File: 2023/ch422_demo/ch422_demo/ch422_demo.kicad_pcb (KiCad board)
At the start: 2 copper layers, 35 x 26 mm, 19 parts, among them J1 ch422, J2 hours, J3 minutes, J4 IIC_Conn

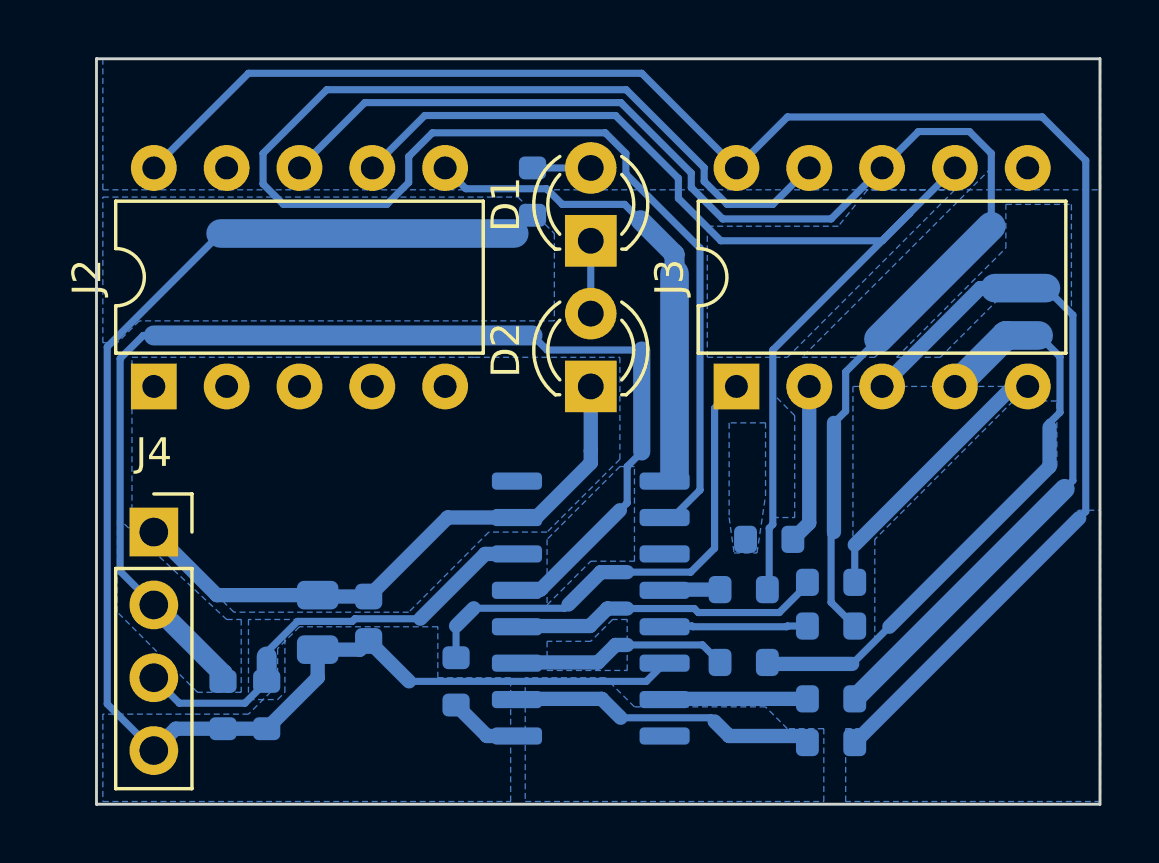
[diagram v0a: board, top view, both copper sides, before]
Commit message: forgot a few weekly commits.
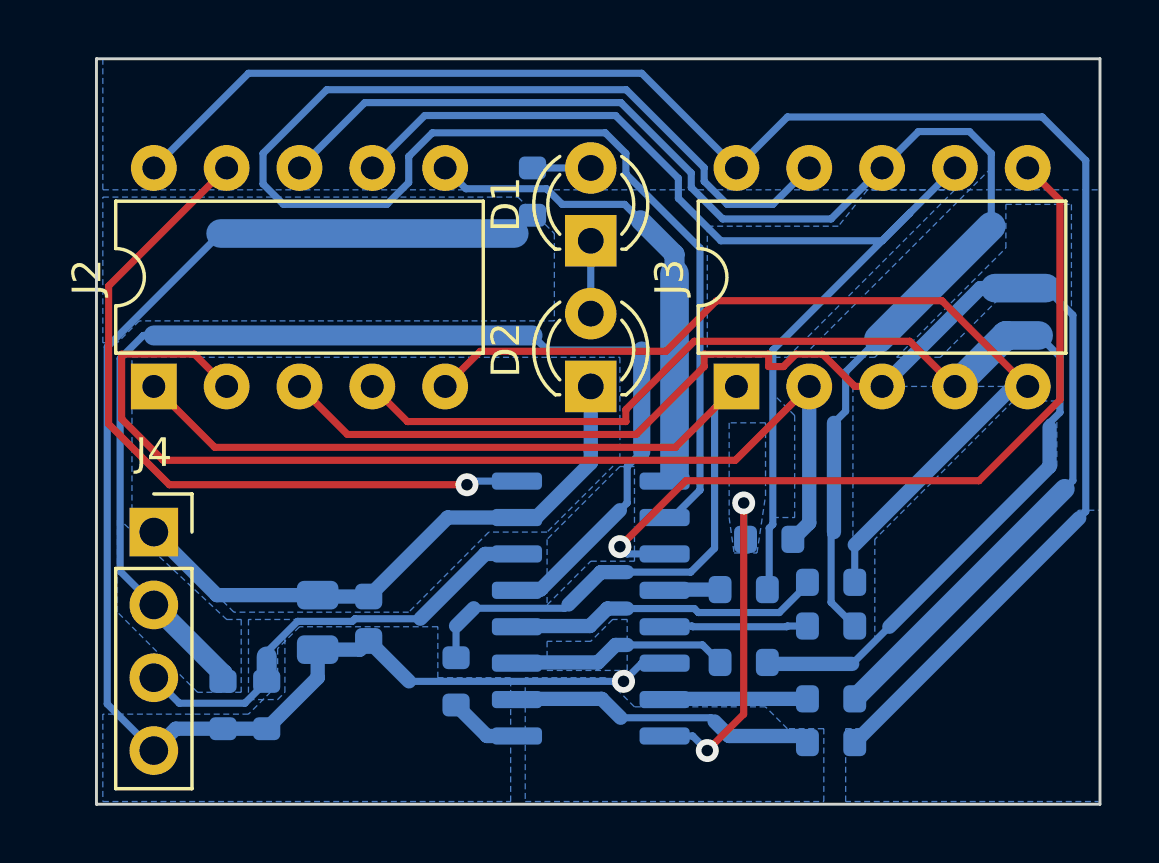
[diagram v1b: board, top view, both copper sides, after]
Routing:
- net /SEG_L_3: track 5.57 -> 37.6 mm
- net /DIG_3: track 0.00 -> 27.7 mm, vias 0 -> 1
- net /DIG_0: track 0.00 -> 25.8 mm, vias 0 -> 1
- net /SEG_L_2: track 25.0 -> 48.5 mm
- net /SEG_L_6: track 21.3 -> 44.2 mm
- net /SEG_L_7: track 9.12 -> 31.9 mm
- net /SEG_L_4: track 17.2 -> 39.3 mm
- net /SEG_3: track 0.00 -> 12.2 mm, vias 0 -> 2
- net VCC: vias 0 -> 1
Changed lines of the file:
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@@
   (gr_rect (start 33.56 17.02) (end 68.56 43.02)
     (stroke (width 0.1) (type default)) (fill none) (layer "Edge.Cuts"))
+  (via (at 51.943 38.735) (size 0.8) (drill 0.4) (layers "F.Cu" "B.Cu") (net 1))
   (segment (start 41.275 37.627853) (end 42.751 37.627853) (width 0.5) (layer "B.Cu") (net 1))
   (segment (start 44.462147 38.735) (end 43.053 37.325853) (width 0.5) (layer "B.Cu") (net 1))
-  (segment (start 52.74 38.735) (end 44.462147 38.735) (width 0.25) (layer "B.Cu") (net 1))
+  (segment (start 52.578 38.1) (end 51.943 38.735) (width 0.25) (layer "B.Cu") (net 1))
   (segment (start 33.935 27.068604) (end 33.935 39.523) (width 0.25) (layer "B.Cu") (net 1))
   (segment (start 36.322 40.386) (end 35.56 41.148) (width 0.5) (layer "B.Cu") (net 1))
-  (segment (start 53.375 38.1) (end 52.74 38.735) (width 0.25) (layer "B.Cu") (net 1))
   (segment (start 41.275 38.608) (end 41.275 37.627853) (width 0.5) (layer "B.Cu") (net 1))
   (segment (start 33.935 39.523) (end 35.56 41.148) (width 0.25) (layer "B.Cu") (net 1))
   (segment (start 42.751 37.627853) (end 43.053 37.325853) (width 0.5) (layer "B.Cu") (net 1))
+  (segment (start 51.943 38.735) (end 44.462147 38.735) (width 0.25) (layer "B.Cu") (net 1))
   (segment (start 37.889604 23.114) (end 33.935 27.068604) (width 0.25) (layer "B.Cu") (net 1))
   (segment (start 48.132 23.114) (end 37.889604 23.114) (width 1) (layer "B.Cu") (net 1))
@@
   (segment (start 39.497 40.386) (end 37.973 40.386) (width 0.5) (layer "B.Cu") (net 1))
   (segment (start 39.497 40.386) (end 41.275 38.608) (width 0.5) (layer "B.Cu") (net 1))
+  (segment (start 53.375 38.1) (end 52.578 38.1) (width 0.25) (layer "B.Cu") (net 1))
   (segment (start 48.225 33.02) (end 48.895 33.02) (width 0.5) (layer "B.Cu") (net 2))
   (segment (start 37.759853 35.727853) (end 35.56 33.528) (width 0.5) (layer "B.Cu") (net 2))
@@
   (segment (start 44.856147 36.550853) (end 47.117 34.29) (width 0.5) (layer "B.Cu") (net 10))
   (segment (start 39.497 38.736) (end 39.497 37.86768) (width 0.7) (layer "B.Cu") (net 10))
+  (segment (start 36.102604 31.877) (end 33.985 29.759396) (width 0.25) (layer "F.Cu") (net 11))
+  (segment (start 33.985 24.943) (end 38.1 20.828) (width 0.25) (layer "F.Cu") (net 11))
+  (segment (start 46.482 31.877) (end 36.102604 31.877) (width 0.25) (layer "F.Cu") (net 11))
+  (segment (start 33.985 29.759396) (end 33.985 24.943) (width 0.25) (layer "F.Cu") (net 11))
+  (via (at 46.482 31.877) (size 0.8) (drill 0.4) (layers "F.Cu" "B.Cu") (net 11))
+  (segment (start 46.609 31.75) (end 46.482 31.877) (width 0.25) (layer "B.Cu") (net 11))
+  (segment (start 48.225 31.75) (end 46.609 31.75) (width 0.25) (layer "B.Cu") (net 11))
   (segment (start 53.721 24.511) (end 53.721 23.839) (width 0.7) (layer "B.Cu") (net 12))
   (segment (start 49.260462 21.553) (end 49.805462 22.098) (width 0.25) (layer "B.Cu") (net 12))
@@
   (segment (start 39.37 20.32) (end 41.5908 18.0992) (width 0.25) (layer "B.Cu") (net 13))
   (segment (start 54.61 32.061751) (end 54.61 23.622) (width 0.25) (layer "B.Cu") (net 13))
+  (segment (start 51.816 34.036) (end 54.115 31.737) (width 0.25) (layer "F.Cu") (net 14))
+  (segment (start 54.115 31.737) (end 64.341991 31.737) (width 0.25) (layer "F.Cu") (net 14))
+  (segment (start 67.165 28.913991) (end 67.165 21.953) (width 0.25) (layer "F.Cu") (net 14))
+  (segment (start 67.165 21.953) (end 66.04 20.828) (width 0.25) (layer "F.Cu") (net 14))
+  (segment (start 64.341991 31.737) (end 67.165 28.913991) (width 0.25) (layer "F.Cu") (net 14))
+  (via (at 51.816 34.036) (size 0.8) (drill 0.4) (layers "F.Cu" "B.Cu") (net 14))
+  (segment (start 52.07 34.29) (end 51.816 34.036) (width 0.25) (layer "B.Cu") (net 14))
+  (segment (start 53.375 34.29) (end 52.07 34.29) (width 0.25) (layer "B.Cu") (net 14))
   (segment (start 53.375 35.534853) (end 55.309 35.534853) (width 0.5) (layer "B.Cu") (net 15))
   (segment (start 57.658 36.804853) (end 58.357 36.804853) (width 0.25) (layer "B.Cu") (net 16))
@@
   (segment (start 53.375 36.804853) (end 54.330853 36.804853) (width 0.25) (layer "B.Cu") (net 16))
   (segment (start 53.375 39.344853) (end 58.357 39.344853) (width 0.5) (layer "B.Cu") (net 17))
+  (segment (start 56.134 39.878) (end 56.134 32.512) (width 0.25) (layer "F.Cu") (net 18))
+  (segment (start 54.864 41.148) (end 56.134 39.878) (width 0.25) (layer "F.Cu") (net 18))
+  (via (at 54.864 41.148) (size 0.8) (drill 0.4) (layers "F.Cu" "B.Cu") (net 18))
+  (via (at 56.134 32.512) (size 0.8) (drill 0.4) (layers "F.Cu" "B.Cu") (net 18))
+  (segment (start 56.134 33.718) (end 56.198 33.782) (width 0.25) (layer "B.Cu") (net 18))
+  (segment (start 53.375 40.64) (end 54.356 40.64) (width 0.25) (layer "B.Cu") (net 18))
+  (segment (start 56.134 32.512) (end 56.134 33.718) (width 0.25) (layer "B.Cu") (net 18))
+  (segment (start 54.356 40.64) (end 54.864 41.148) (width 0.25) (layer "B.Cu") (net 18))
+  (segment (start 55.88 28.448) (end 53.755 30.573) (width 0.25) (layer "F.Cu") (net 19))
+  (segment (start 53.755 30.573) (end 37.685 30.573) (width 0.25) (layer "F.Cu") (net 19))
+  (segment (start 37.685 30.573) (end 35.56 28.448) (width 0.25) (layer "F.Cu") (net 19))
   (segment (start 52.07 34.925) (end 54.286751 34.925) (width 0.25) (layer "B.Cu") (net 19))
   (segment (start 46.717125 36.185) (end 49.893249 36.185) (width 0.25) (layer "B.Cu") (net 19))
@@
   (segment (start 46.101 37.91) (end 46.101 36.801125) (width 0.25) (layer "B.Cu") (net 19))
   (segment (start 55.118 29.21) (end 55.88 28.448) (width 0.25) (layer "B.Cu") (net 19))
+  (segment (start 38.1 28.448) (end 36.975 27.323) (width 0.25) (layer "F.Cu") (net 20))
+  (segment (start 34.435 29.573) (end 35.885 31.023) (width 0.25) (layer "F.Cu") (net 20))
+  (segment (start 35.885 31.023) (end 55.845 31.023) (width 0.25) (layer "F.Cu") (net 20))
+  (segment (start 55.845 31.023) (end 58.42 28.448) (width 0.25) (layer "F.Cu") (net 20))
+  (segment (start 34.435 27.323) (end 34.435 29.573) (width 0.25) (layer "F.Cu") (net 20))
+  (segment (start 36.975 27.323) (end 34.435 27.323) (width 0.25) (layer "F.Cu") (net 20))
   (segment (start 58.42 28.448) (end 58.42 33.21) (width 0.5) (layer "B.Cu") (net 20))
   (segment (start 58.42 33.21) (end 57.848 33.782) (width 0.5) (layer "B.Cu") (net 20))
+  (segment (start 60.010991 28.448) (end 60.96 28.448) (width 0.25) (layer "F.Cu") (net 21))
+  (segment (start 57.954009 27.323) (end 58.885991 27.323) (width 0.25) (layer "F.Cu") (net 21))
+  (segment (start 52.387 30.123) (end 54.755 27.755) (width 0.25) (layer "F.Cu") (net 21))
+  (segment (start 58.885991 27.323) (end 60.010991 28.448) (width 0.25) (layer "F.Cu") (net 21))
+  (segment (start 57.005 27.323) (end 57.005 27.755) (width 0.25) (layer "F.Cu") (net 21))
+  (segment (start 57.005 27.755) (end 57.522009 27.755) (width 0.25) (layer "F.Cu") (net 21))
+  (segment (start 54.755 27.323) (end 57.005 27.323) (width 0.25) (layer "F.Cu") (net 21))
+  (segment (start 57.522009 27.755) (end 57.954009 27.323) (width 0.25) (layer "F.Cu") (net 21))
+  (segment (start 40.64 28.448) (end 42.315 30.123) (width 0.25) (layer "F.Cu") (net 21))
+  (segment (start 54.755 27.755) (end 54.755 27.323) (width 0.25) (layer "F.Cu") (net 21))
+  (segment (start 42.315 30.123) (end 52.387 30.123) (width 0.25) (layer "F.Cu") (net 21))
   (segment (start 64.389 25.019) (end 60.96 28.448) (width 0.5) (layer "B.Cu") (net 21))
   (segment (start 67.615 31.736853) (end 67.615 25.959) (width 0.25) (layer "B.Cu") (net 21))
@@
   (segment (start 67.615 25.959) (end 66.675 25.019) (width 0.25) (layer "B.Cu") (net 21))
   (segment (start 64.897 25.019) (end 64.389 25.019) (width 0.5) (layer "B.Cu") (net 21))
+  (segment (start 63.5 28.448) (end 61.925 26.873) (width 0.25) (layer "F.Cu") (net 22))
+  (segment (start 52.025 29.255) (end 52.025 29.673) (width 0.25) (layer "F.Cu") (net 22))
+  (segment (start 52.025 29.673) (end 44.405 29.673) (width 0.25) (layer "F.Cu") (net 22))
+  (segment (start 54.407 26.873) (end 52.025 29.255) (width 0.25) (layer "F.Cu") (net 22))
+  (segment (start 44.405 29.673) (end 43.18 28.448) (width 0.25) (layer "F.Cu") (net 22))
+  (segment (start 61.925 26.873) (end 54.407 26.873) (width 0.25) (layer "F.Cu") (net 22))
   (segment (start 66.421 26.67) (end 67.165 27.414) (width 0.25) (layer "B.Cu") (net 22))
   (segment (start 65.278 26.67) (end 63.5 28.448) (width 1) (layer "B.Cu") (net 22))
@@
   (segment (start 66.802 29.718) (end 66.802 29.8704) (width 0.3) (layer "B.Cu") (net 22))
   (segment (start 67.165 27.414) (end 67.165 29.355) (width 0.25) (layer "B.Cu") (net 22))
+  (segment (start 55.185604 25.458) (end 63.05 25.458) (width 0.25) (layer "F.Cu") (net 23))
+  (segment (start 46.945 27.223) (end 53.420604 27.223) (width 0.25) (layer "F.Cu") (net 23))
+  (segment (start 63.05 25.458) (end 66.04 28.448) (width 0.25) (layer "F.Cu") (net 23))
+  (segment (start 45.72 28.448) (end 46.945 27.223) (width 0.25) (layer "F.Cu") (net 23))
+  (segment (start 53.420604 27.223) (end 55.185604 25.458) (width 0.25) (layer "F.Cu") (net 23))
   (segment (start 60.007 35.280853) (end 60.007 33.971604) (width 0.25) (layer "B.Cu") (net 23))
   (segment (start 60.007 33.971604) (end 65.530604 28.448) (width 0.5) (layer "B.Cu") (net 23))
@@
         (xy 64.77 23.368)
         (xy 64.77 20.828)
-        (xy 58.166 27.432)
-        (xy 58.166 27.432)
-      )
-    )
+      )
+    )
